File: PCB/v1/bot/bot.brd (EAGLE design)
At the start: 35.9 x 32.1 mm, 3 parts, among them J1 SMA-J-P-H-ST-EM1

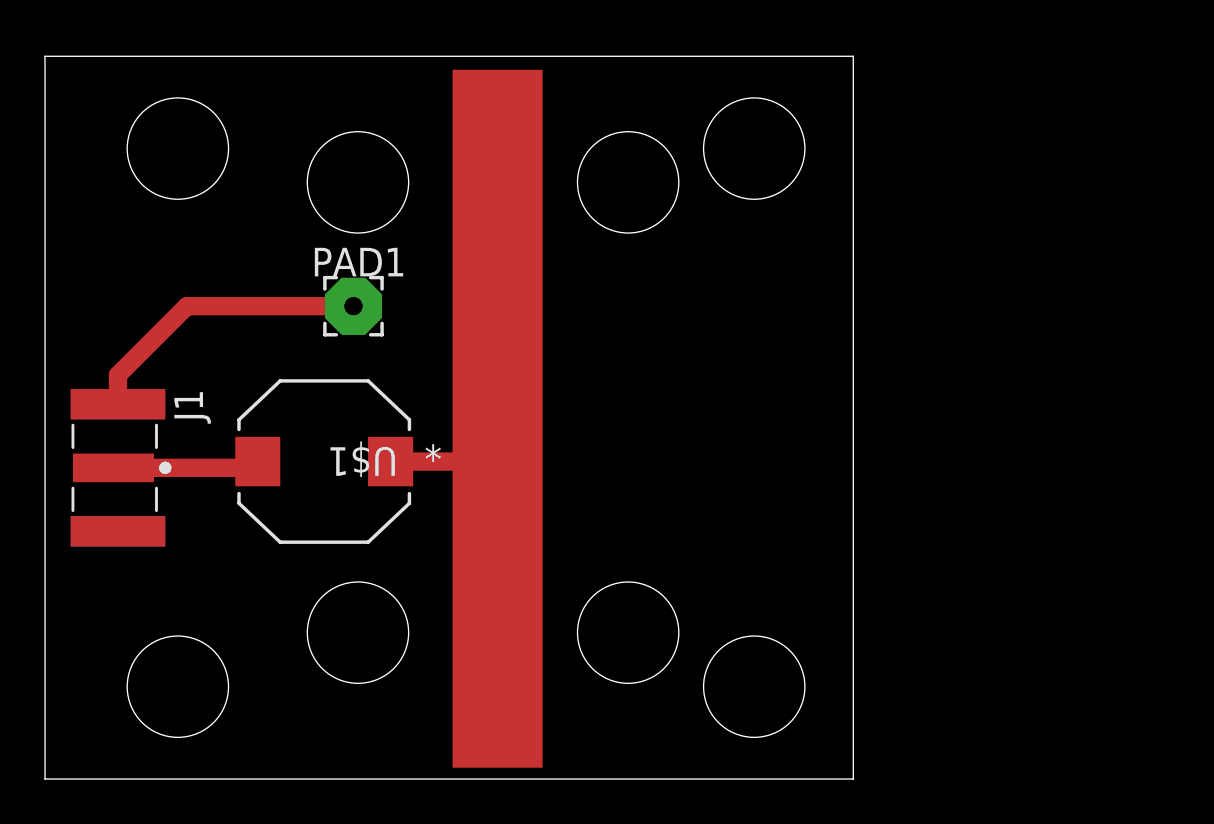
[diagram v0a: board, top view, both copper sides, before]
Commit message: updates
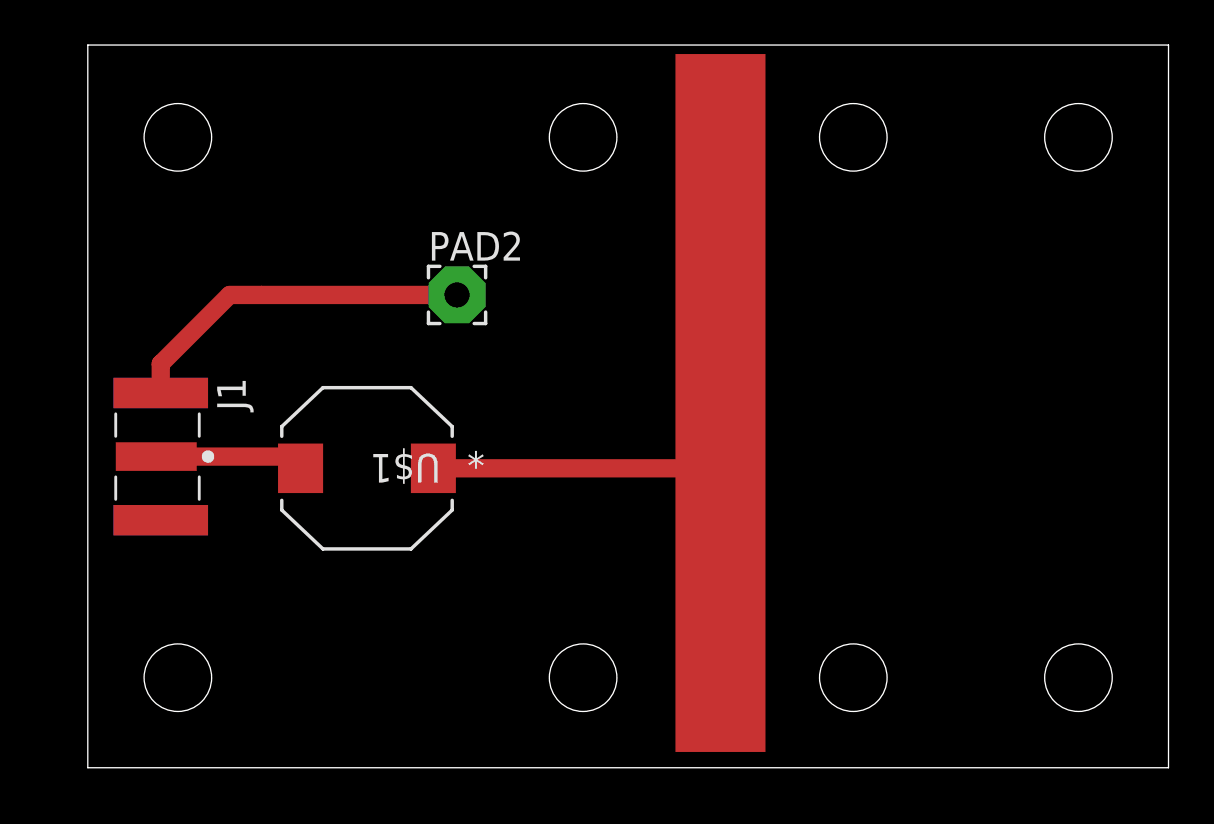
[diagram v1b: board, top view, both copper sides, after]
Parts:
- removed PAD1: (no value), wirepad:2,54/0,8
- added PAD2: (no value), wirepad:2,54/1,1
- moved J1 1.96 mm to (3.04, 13.8)
- moved U$1 1.92 mm to (12.4, 13.3)
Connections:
- net GND: now also PAD2.1; no longer PAD1.1
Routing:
- net CRYSTAL: track 5.08 -> 11.6 mm
- net GND: track 13.0 -> 15.7 mm
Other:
- board size 35.9 x 32.1 mm -> 48 x 32.1 mm
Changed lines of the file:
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@@
 <?xml version="1.0" encoding="utf-8"?>
 <!DOCTYPE eagle SYSTEM "eagle.dtd">
-<eagle version="9.3.0">
+<eagle version="9.3.2">
 <drawing>
 <settings>
@@
 <board>
 <plain>
-<wire x1="-1.9" y1="-0.5" x2="34" y2="-0.5" width="0" layer="20"/>
-<wire x1="34" y1="-0.5" x2="34" y2="31.6" width="0" layer="20"/>
-<wire x1="34" y1="31.6" x2="-1.9" y2="31.6" width="0" layer="20"/>
-<wire x1="-1.9" y1="31.6" x2="-1.9" y2="-0.5" width="0" layer="20"/>
-<rectangle x1="16.2" y1="0" x2="20.2" y2="31" layer="1" rot="R180"/>
-<hole x="12" y="6" drill="4.5"/>
-<hole x="12" y="26" drill="4.5"/>
-<hole x="24" y="26" drill="4.5"/>
-<hole x="4" y="27.5" drill="4.5"/>
-<hole x="4" y="3.6" drill="4.5"/>
-<hole x="29.6" y="3.6" drill="4.5"/>
-<hole x="29.6" y="27.5" drill="4.5"/>
-<hole x="24" y="6" drill="4.5"/>
+<wire x1="0" y1="0" x2="48" y2="0" width="0" layer="20"/>
+<wire x1="48" y1="0" x2="48" y2="32.1" width="0" layer="20"/>
+<wire x1="48" y1="32.1" x2="0" y2="32.1" width="0" layer="20"/>
+<wire x1="0" y1="32.1" x2="0" y2="0" width="0" layer="20"/>
+<rectangle x1="26.1" y1="0.7" x2="30.1" y2="31.7" layer="1" rot="R180"/>
+<hole x="22" y="28" drill="3"/>
+<hole x="34" y="28" drill="3"/>
+<hole x="4" y="28" drill="3"/>
+<hole x="4" y="4" drill="3"/>
+<hole x="44" y="4" drill="3"/>
+<hole x="44" y="28" drill="3"/>
+<hole x="22" y="4" drill="3"/>
+<hole x="34" y="4" drill="3"/>
+<dimension x1="0" y1="32.1" x2="0" y2="0" x3="38.1" y3="16.05" textsize="1.778" layer="1"/>
+<dimension x1="48" y1="32.1" x2="0" y2="32.1" x3="24" y3="22.4" textsize="1.778" layer="1"/>
+<dimension x1="16.7" y1="10.2" x2="24.4" y2="9.4" x3="24.4" y3="9.8" textsize="1.778" layer="255" dtype="vertical"/>
+<dimension x1="16" y1="15.9" x2="18.5" y2="15.5" x3="18.5" y3="15.7" textsize="1.778" layer="255" dtype="vertical"/>
+<dimension x1="34" y1="28" x2="35.1" y2="32.2" x3="35.7" y3="30.1" textsize="1.778" layer="255" dtype="vertical"/>
+<dimension x1="35.2" y1="30" x2="34.8" y2="30.1" x3="34.8" y3="30.05" textsize="1.778" layer="255" dtype="vertical"/>
+<dimension x1="34" y1="28" x2="34.2" y2="32.1" x3="34.3" y3="30.05" textsize="1.778" layer="255" dtype="vertical"/>
+<dimension x1="21.973915625" y1="29.499771875" x2="22.026084375" y2="26.500228125" x3="33.5" y3="28.200009375" textsize="1.778" layer="255" dtype="diameter"/>
+<dimension x1="22" y1="28" x2="34" y2="28" x3="28" y3="28" textsize="1.778" layer="255"/>
+<dimension x1="23.5" y1="28" x2="20.5" y2="28" x3="22" y3="4" textsize="1.778" layer="255" dtype="diameter"/>
+<dimension x1="22" y1="4" x2="22" y2="28" x3="24.7" y3="16" textsize="1.778" layer="255"/>
 </plain>
 <attributes>
@@
 </autorouter>
 <elements>
-<element name="J1" library="SMA-J-P-H-ST-EM1" package="SMA-J-P-H-ST-EM1" value="SMA-J-P-H-ST-EM1" x="1.14" y="13.32" smashed="yes" rot="R270">
-<attribute name="DESCRIPTION" value=" Connector SMA F 50Ohm Solder ST Edge Mount Gold Over Nickel Tray " x="1.14" y="13.32" size="1.778" layer="27" rot="R270" display="off"/>
-<attribute name="DIGI-KEY_PART_NUMBER" value="SAM8857-ND" x="1.14" y="13.32" size="1.778" layer="27" rot="R270" display="off"/>
-<attribute name="DIGI-KEY_PURCHASE_URL" value="https://www.digikey.com/product-detail/en/samtec-inc/SMA-J-P-H-ST-EM1/SAM8857-ND/2602450?utm_source=snapeda&amp;utm_medium=aggregator&amp;utm_campaign=symbol" x="1.14" y="13.32" size="1.778" layer="27" rot="R270" display="off"/>
-<attribute name="MF" value="Samtec" x="1.14" y="13.32" size="1.778" layer="27" rot="R270" display="off"/>
-<attribute name="MP" value="SMA-J-P-H-ST-EM1" x="1.14" y="13.32" size="1.778" layer="27" rot="R270" display="off"/>
-<attribute name="NAME" x="3.84466875" y="16.82605" size="1.2722" layer="25" rot="R270"/>
-<attribute name="PACKAGE" value="None" x="1.14" y="13.32" size="1.778" layer="27" rot="R270" display="off"/>
-<attribute name="VALUE" x="-11.8627" y="16.720709375" size="1.270259375" layer="27" rot="R270"/>
+<element name="J1" library="SMA-J-P-H-ST-EM1" package="SMA-J-P-H-ST-EM1" value="SMA-J-P-H-ST-EM1" x="3.04" y="13.82" smashed="yes" rot="R270">
+<attribute name="DESCRIPTION" value=" Connector SMA F 50Ohm Solder ST Edge Mount Gold Over Nickel Tray " x="3.04" y="13.82" size="1.778" layer="27" rot="R270" display="off"/>
+<attribute name="DIGI-KEY_PART_NUMBER" value="SAM8857-ND" x="3.04" y="13.82" size="1.778" layer="27" rot="R270" display="off"/>
+<attribute name="DIGI-KEY_PURCHASE_URL" value="https://www.digikey.com/product-detail/en/samtec-inc/SMA-J-P-H-ST-EM1/SAM8857-ND/2602450?utm_source=snapeda&amp;utm_medium=aggregator&amp;utm_campaign=symbol" x="3.04" y="13.82" size="1.778" layer="27" rot="R270" display="off"/>
+<attribute name="MF" value="Samtec" x="3.04" y="13.82" size="1.778" layer="27" rot="R270" display="off"/>
+<attribute name="MP" value="SMA-J-P-H-ST-EM1" x="3.04" y="13.82" size="1.778" layer="27" rot="R270" display="off"/>
+<attribute name="NAME" x="5.74466875" y="17.32605" size="1.2722" layer="25" rot="R270"/>
+<attribute name="PACKAGE" value="None" x="3.04" y="13.82" size="1.778" layer="27" rot="R270" display="off"/>
+<attribute name="VALUE" x="-9.9627" y="17.220709375" size="1.270259375" layer="27" rot="R270"/>
 </element>
-<element name="PAD1" library="wirepad" library_urn="urn:adsk.eagle:library:412" package="2,54/0,8" package3d_urn="urn:adsk.eagle:package:30838/1" value="" x="11.8" y="20.5" smashed="yes">
-<attribute name="NAME" x="9.93" y="21.824" size="1.27" layer="25" ratio="10"/>
-<attribute name="VALUE" x="11.8" y="21.1" size="0.0254" layer="27"/>
+<element name="U$1" library="new_inductor" package="IND_7030" value="INDUCTOR" x="12.4" y="13.3" smashed="yes" rot="R180">
+<attribute name="NAME" x="15.6766" y="13.935" size="1.27" layer="25" ratio="6" rot="SR180"/>
 </element>
-<element name="U$1" library="new_inductor" package="IND_7030" value="INDUCTOR" x="10.5" y="13.6" smashed="yes" rot="R180">
-<attribute name="NAME" x="13.7766" y="14.235" size="1.27" layer="25" ratio="6" rot="SR180"/>
+<element name="PAD2" library="wirepad" library_urn="urn:adsk.eagle:library:412" package="2,54/1,1" package3d_urn="urn:adsk.eagle:package:30836/1" value="" x="16.4" y="21" smashed="yes">
+<attribute name="NAME" x="15.13" y="22.524" size="1.27" layer="25" ratio="10"/>
+<attribute name="VALUE" x="16.4" y="22" size="0.0254" layer="27"/>
 </element>
 </elements>
@@
 <contactref element="J1" pad="3_2"/>
 <contactref element="J1" pad="2_1"/>
-<contactref element="PAD1" pad="1"/>
-<wire x1="11.8" y1="20.5" x2="4.4" y2="20.5" width="0.8128" layer="1"/>
-<wire x1="4.4" y1="20.5" x2="1.34" y2="17.44" width="0.8128" layer="1"/>
-<wire x1="1.34" y1="17.44" x2="1.34" y2="16.145" width="0.8128" layer="1"/>
-<wire x1="1.34" y1="16.145" x2="1.34" y2="16.145" width="0" layer="19" extent="1-16"/>
-<wire x1="1.34" y1="10.495" x2="1.34" y2="16.145" width="0" layer="19" extent="1-16"/>
-<wire x1="1.34" y1="10.495" x2="1.34" y2="10.495" width="0" layer="19" extent="1-16"/>
+<wire x1="3.24" y1="17.94" x2="6.3" y2="21" width="0.8128" layer="1"/>
+<wire x1="3.24" y1="17.94" x2="3.24" y2="16.645" width="0.8128" layer="1"/>
+<contactref element="PAD2" pad="1"/>
+<wire x1="6.3" y1="21" x2="7.7" y2="21" width="0.812853125" layer="1"/>
+<wire x1="7.7" y1="21" x2="16.4" y2="21" width="0.8128" layer="1"/>
+<wire x1="3.24" y1="16.645" x2="3.24" y2="16.645" width="0" layer="19" extent="1-16"/>
+<wire x1="3.24" y1="10.995" x2="3.24" y2="16.645" width="0" layer="19" extent="1-16"/>
+<wire x1="3.24" y1="10.995" x2="3.24" y2="10.995" width="0" layer="19" extent="1-16"/>
 </signal>
 <signal name="2L">
 <contactref element="J1" pad="1"/>
 <contactref element="U$1" pad="2"/>
-<wire x1="1.14" y1="13.32" x2="7.27" y2="13.32" width="0.8128" layer="1"/>
-<wire x1="7.27" y1="13.32" x2="7.55" y2="13.6" width="0.1524" layer="1"/>
+<wire x1="9.45" y1="13.3" x2="8.93" y2="13.82" width="0.8128" layer="1"/>
+<wire x1="8.93" y1="13.82" x2="3.04" y2="13.82" width="0.8128" layer="1"/>
 </signal>
 <signal name="CRYSTAL">
 <contactref element="U$1" pad="1"/>
-<wire x1="13.45" y1="13.6" x2="18.5286" y2="13.6" width="0.8128" layer="1"/>
+<wire x1="15.35" y1="13.3" x2="26.9286" y2="13.3" width="0.8128" layer="1"/>
 </signal>
 </signals>
